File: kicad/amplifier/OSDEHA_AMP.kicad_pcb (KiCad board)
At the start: 2 copper layers, 90 parts, among them J1 INPUT, J2 HEATERS DC, J3 PSU HV, J4 OUTPUT, J5 DHT FIL2, J6 DHT FIL1, Q1 DN2540N5-G, Q10 DN2540, Q2 DN2540N5-G, Q3 STF3LN80K5, Q4 STF3LN80K5, Q5 AOT1N60, Q6 IXTP3N100D2, Q7 AOT1N60, Q8 IXTP3N100D2, Q9 DN2540, SW1 SW_DPDT_x2, U1 6E5P, U2 6E5P, U3 801A, U4 801A

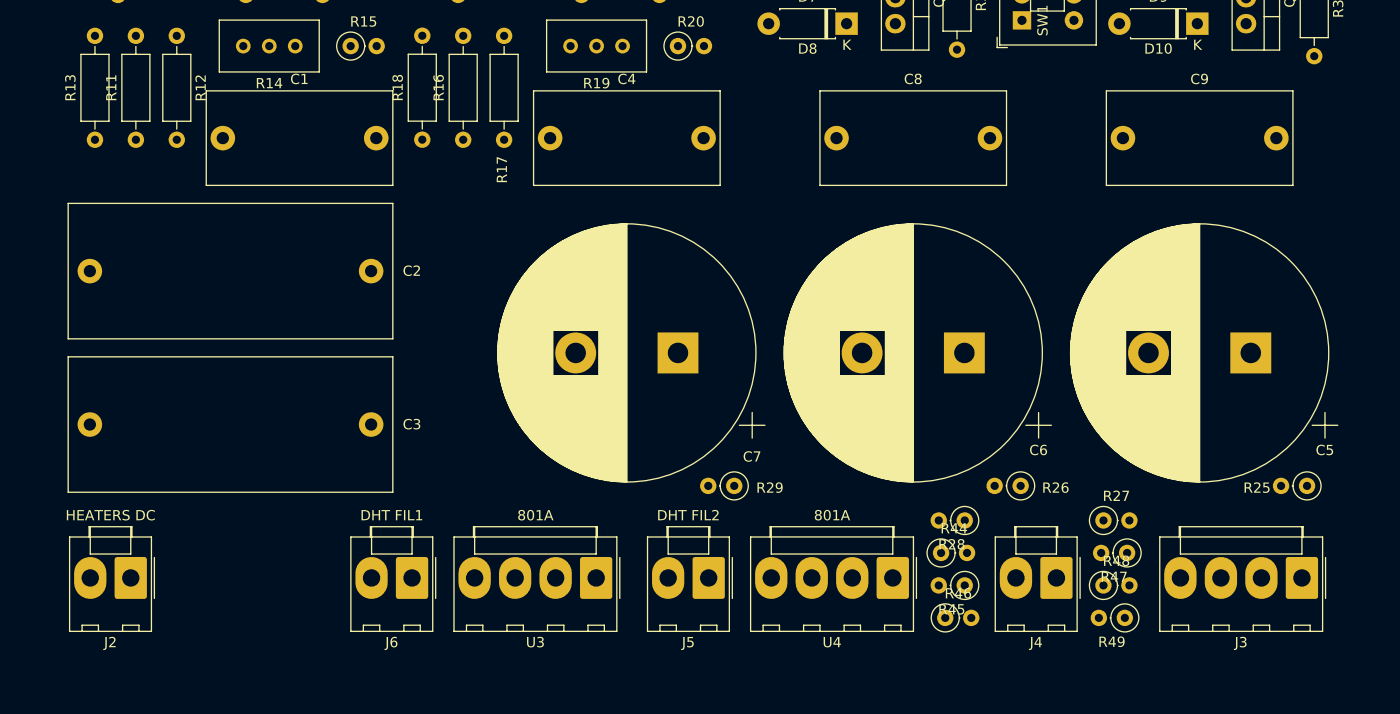
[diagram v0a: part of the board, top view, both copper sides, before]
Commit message: HV filter caps
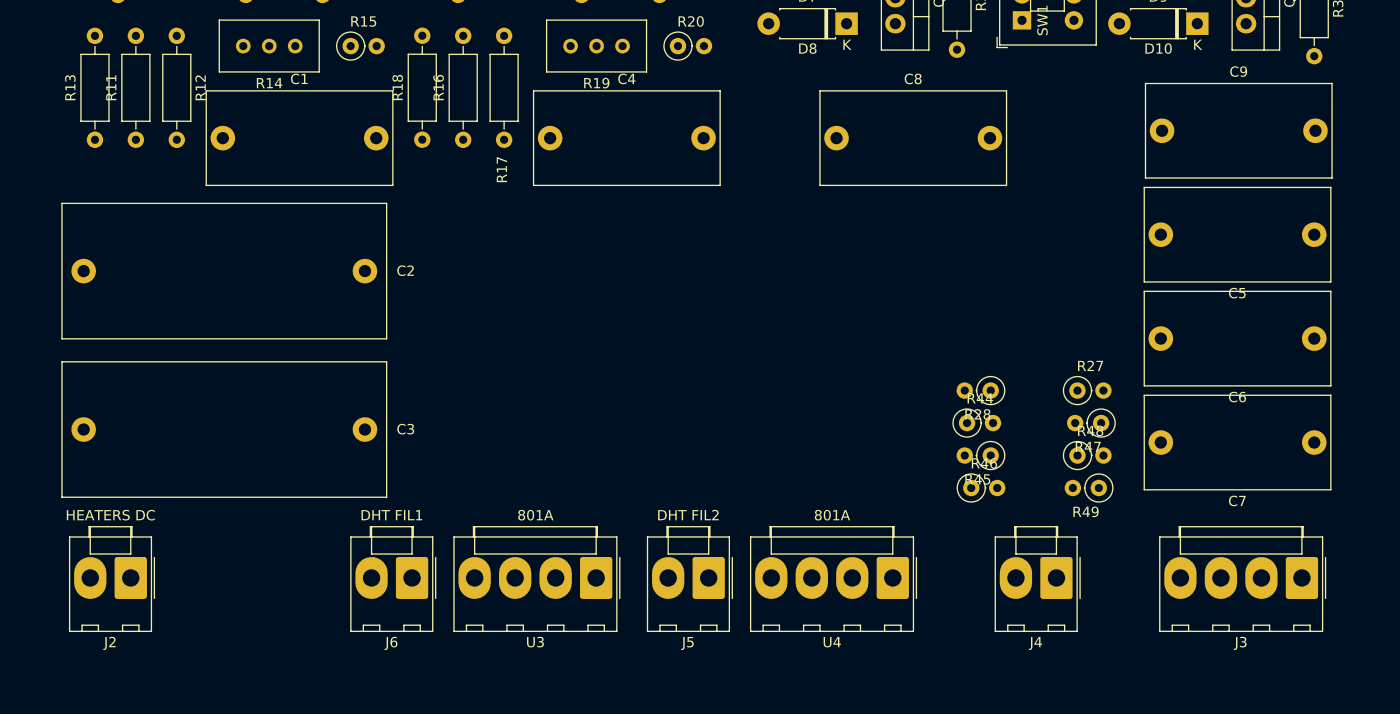
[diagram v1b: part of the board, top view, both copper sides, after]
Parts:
- removed R25, R26, R29: 1M, Resistor_THT:R_Axial_DIN0207_L6.3mm_D2.5mm_P2.54mm_Vertical
- C5, C6, C7: value 51u -> 220n 630 V; footprint Capacitor_THT:CP_Radial_D25.0mm_P10.00mm_SnapIn -> Capacitor_THT:C_Rect_L18.0mm_W9.0mm_P15.00mm_FKS3_FKP3
- moved C7 62.8 mm to (250.7, 111.8)
- moved C6 34.2 mm to (250.7, 101.6)
- moved C5 13.1 mm to (250.7, 91.4)
- moved R44 13.0 mm to (216.8, 109.9)
- moved R45 13.0 mm to (219.1, 113.0)
- moved R46 13.0 mm to (217.2, 116.2)
- moved R47 13.0 mm to (229.9, 109.9)
- moved R48 13.0 mm to (227.6, 113.0)
- moved R49 13.0 mm to (229.6, 116.2)
- moved R27 13.0 mm to (227.6, 106.7)
- moved R28 13.0 mm to (219.1, 106.7)
- moved C9 3.89 mm to (235.8, 81.3)
- moved C3 0.78 mm to (157.9, 110.5)
- moved C2 0.60 mm to (157.9, 95.0)
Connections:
- C5 pad 1: /Dual_Gyrator/+HV -> GND
- C5 pad 2: GND -> /Dual_Gyrator/+HV

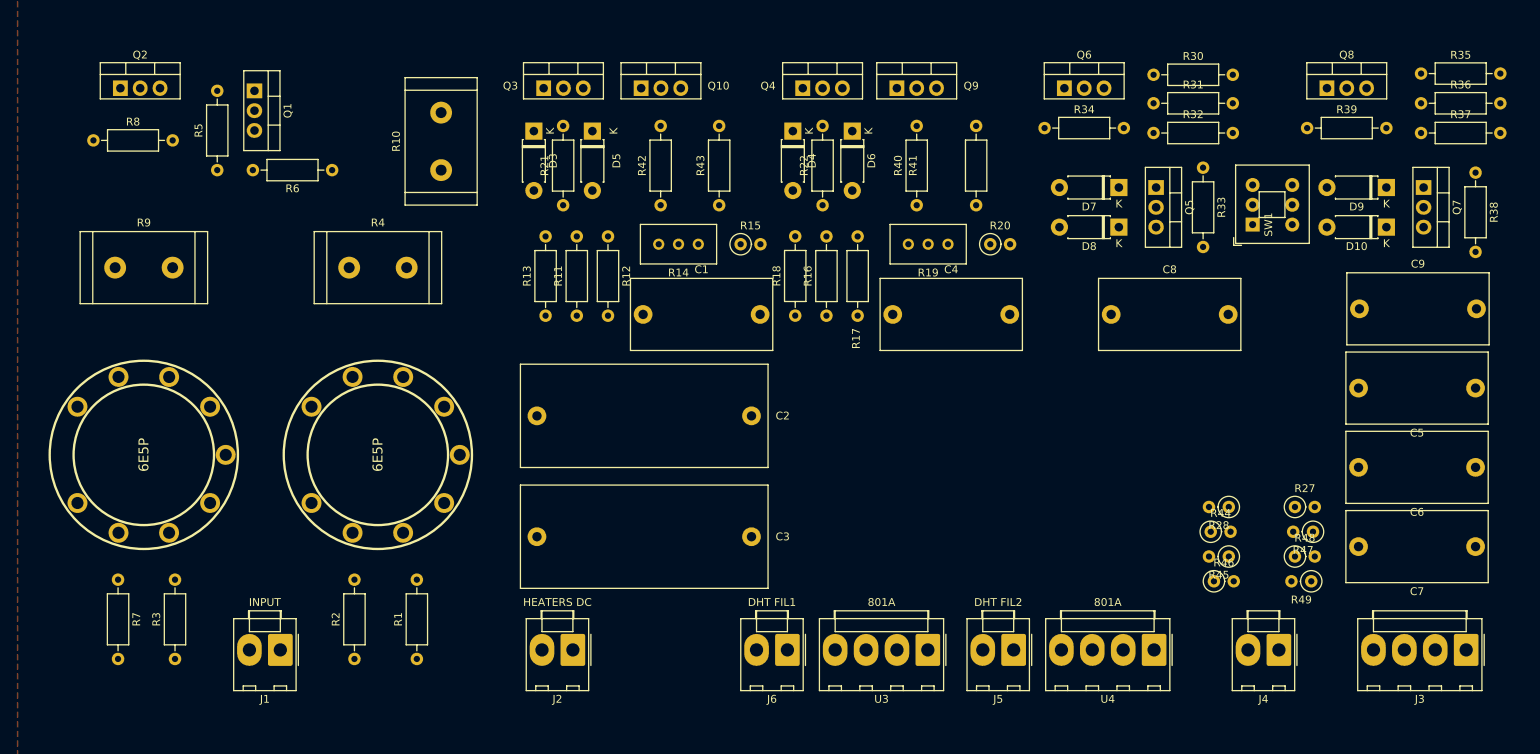
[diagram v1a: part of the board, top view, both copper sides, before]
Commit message: PCB rearrange
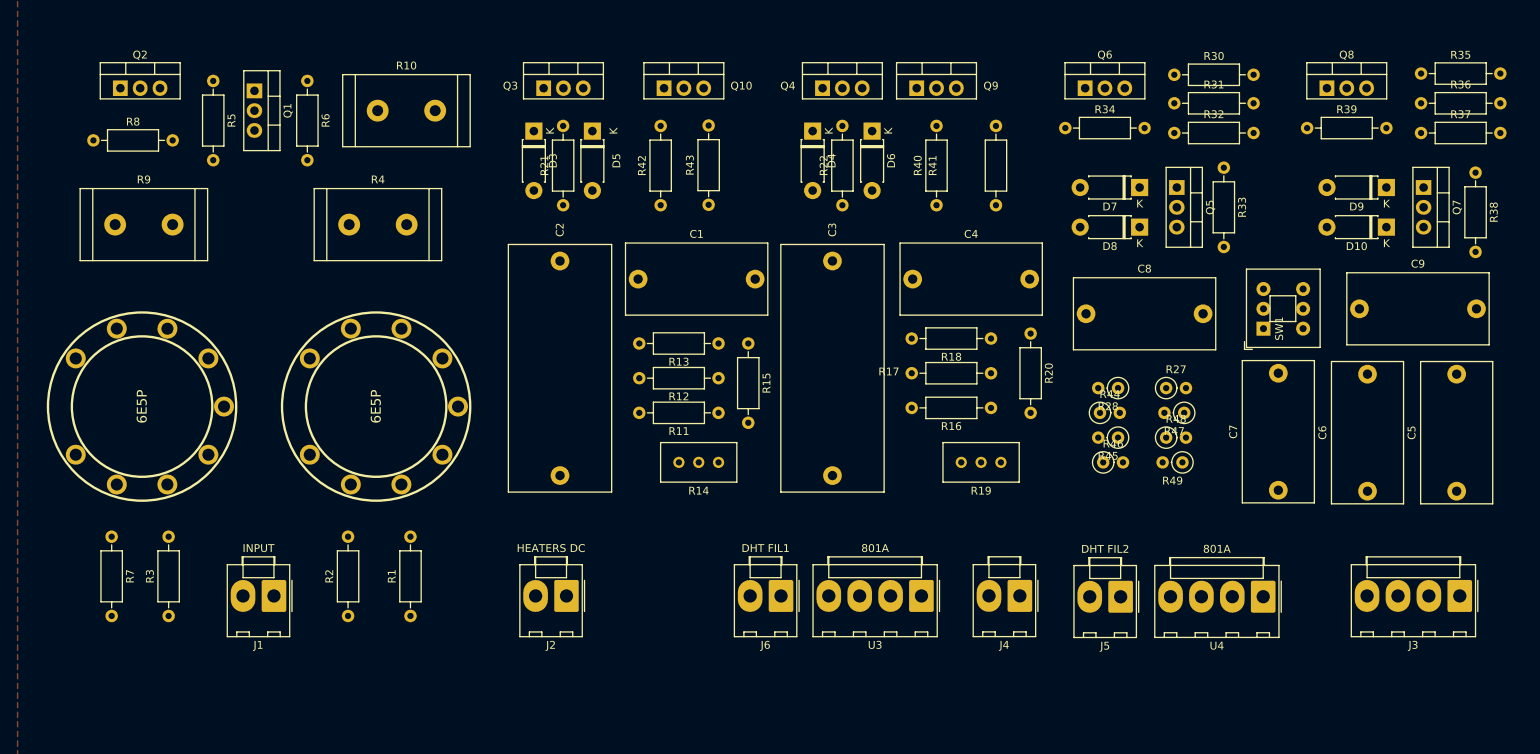
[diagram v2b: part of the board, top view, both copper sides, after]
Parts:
- R15, R20: footprint Resistor_THT:R_Axial_DIN0207_L6.3mm_D2.5mm_P2.54mm_Vertical -> Resistor_THT:R_Axial_DIN0207_L6.3mm_D2.5mm_P10.16mm_Horizontal
- moved C3 36.8 mm to (168.3, 75.2), turned to -90 degrees
- moved J4 33.9 mm to (192.3, 118.1)
- moved C2 31.6 mm to (133.3, 75.2), turned to -90 degrees
- moved R19 28.8 mm to (184.8, 101.0)
- moved R14 28.1 mm to (148.6, 101.0)
- moved C7 26.3 mm to (225.4, 104.5), turned to 90 degrees
- moved R18 25.3 mm to (188.6, 85.1), turned to 180 degrees
- moved R17 24.5 mm to (188.6, 89.5), turned to 180 degrees
- moved R16 24.2 mm to (188.6, 94.0), turned to 180 degrees
- moved R12 23.0 mm to (153.7, 90.2), turned to 180 degrees
- moved R27 22.5 mm to (211.0, 91.4)
- moved R48 22.5 mm to (211.0, 97.8)
- moved R49 22.5 mm to (213.1, 101.0)
- moved R47 22.5 mm to (213.4, 94.6)
- moved R13 22.5 mm to (153.7, 85.7), turned to 180 degrees
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
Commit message: pcb
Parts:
- removed H5: VENTILATION, MountingHole:MountingHole_5mm
- moved H4 222.6 mm to (251.5, 116.8)
- moved H3 193.8 mm to (225.4, 67.9)
- moved H1 64.9 mm to (95.2, 70.9)
- moved H2 64.4 mm to (70.5, 116.8)
- moved J2 9.65 mm to (125.1, 114.8)
- moved J3 7.86 mm to (241.5, 114.8)
- moved J5 3.90 mm to (203.2, 114.8)
- moved U4 3.89 mm to (221.5, 114.8)
- moved J6 3.81 mm to (159.7, 114.8)
- moved U3 3.81 mm to (177.7, 114.8)
- moved J4 3.80 mm to (190.3, 114.8)
- moved R7 3.42 mm to (79.1, 109.2)
- moved J1 3.29 mm to (97.2, 114.8)
- moved R1 2.96 mm to (111.5, 119.4)
- moved R3 2.29 mm to (85.1, 119.4)
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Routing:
- removed copper zone on F.Cu, net GND
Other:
- board outline added: 189.9 x 72.4 mm

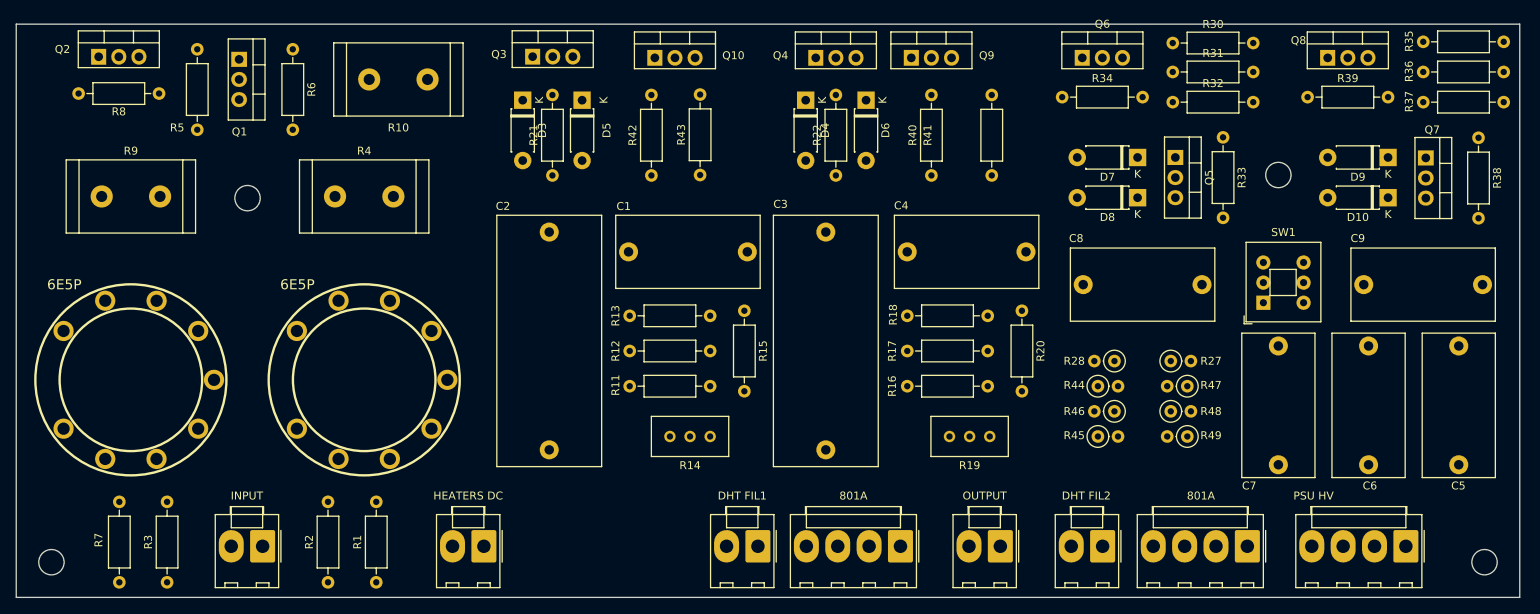
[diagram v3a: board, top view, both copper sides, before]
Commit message: pcb
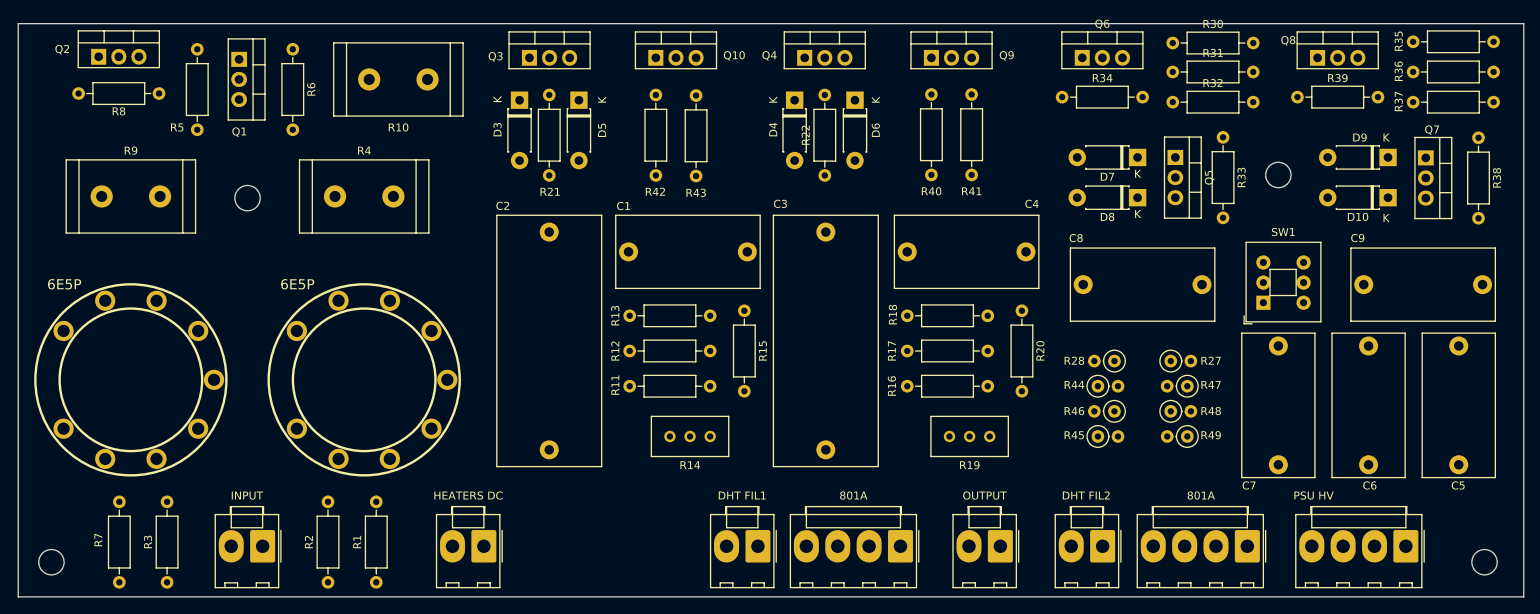
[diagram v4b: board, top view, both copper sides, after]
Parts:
- moved R40 10.2 mm to (181.6, 57.8), turned to -90 degrees
- moved R42 10.2 mm to (146.8, 57.8), turned to -90 degrees
- moved R41 2.54 mm to (186.7, 67.9)
- moved Q9 2.54 mm to (181.6, 53.1)
- moved D4 1.40 mm to (164.3, 58.5)
- moved D6 1.40 mm to (172.0, 58.5)
- moved Q4 1.40 mm to (165.6, 53.1)
- moved R22 1.40 mm to (168.1, 68.0)
- moved Q8 1.28 mm to (230.4, 53.1)
- moved R39 1.28 mm to (227.8, 58.1)
- moved R35 1.28 mm to (242.4, 51.1)
- moved R36 1.28 mm to (242.4, 54.9)
- moved R37 1.28 mm to (242.4, 58.7)
- moved R43 0.52 mm to (151.9, 68.1)
- moved Q3 0.43 mm to (130.8, 53.1)
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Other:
- board size 189.9 x 72.4 mm -> 190.1 x 72.4 mm
